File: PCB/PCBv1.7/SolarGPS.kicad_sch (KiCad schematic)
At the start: 38 parts, among them J1 Conn_01x10_Female, J2 GND, J3 GND, J4 Solar1+, J5 Solar2+, J6 Conn_02x03_Odd_Even, J7 Screw_Terminal_01x01, J8 Conn_01x04_Male, SW1 SW_Push, U1 TPS63802, U2 SAM-M10Q, U3 STM32L071KBTx, U4 MAX40200AUK, Y1 32.768

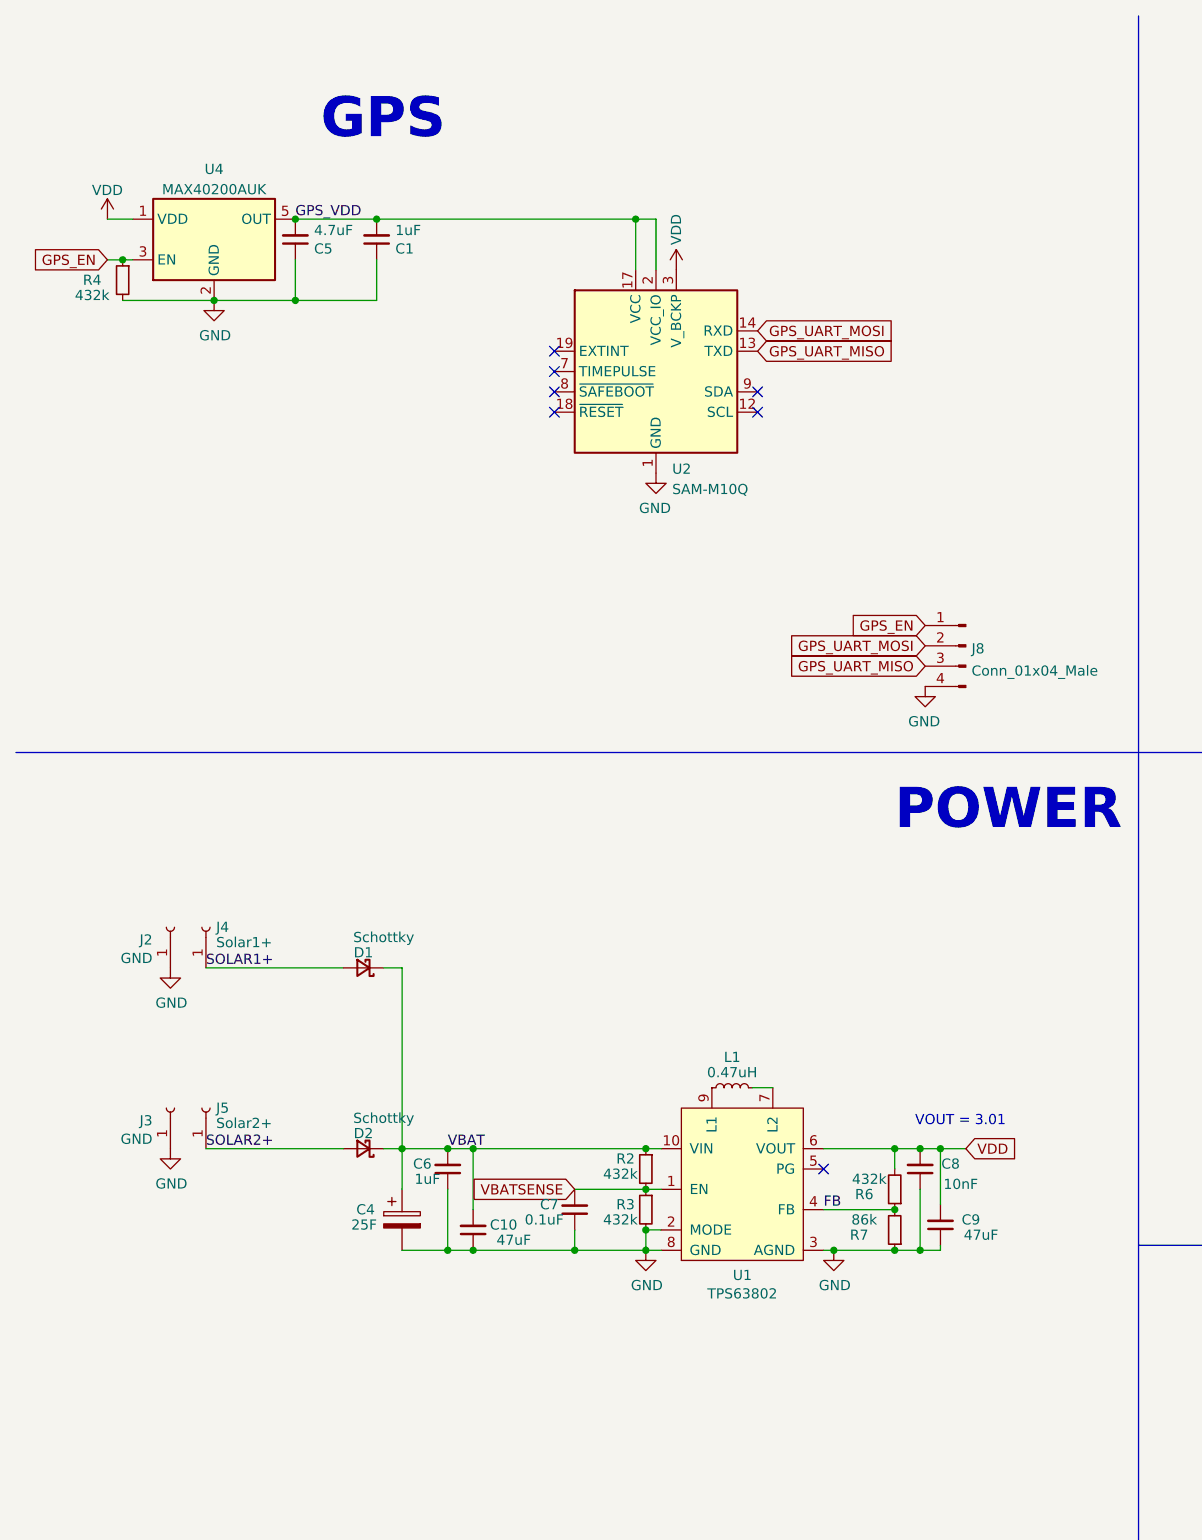
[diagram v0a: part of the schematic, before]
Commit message: Submit board 1.7
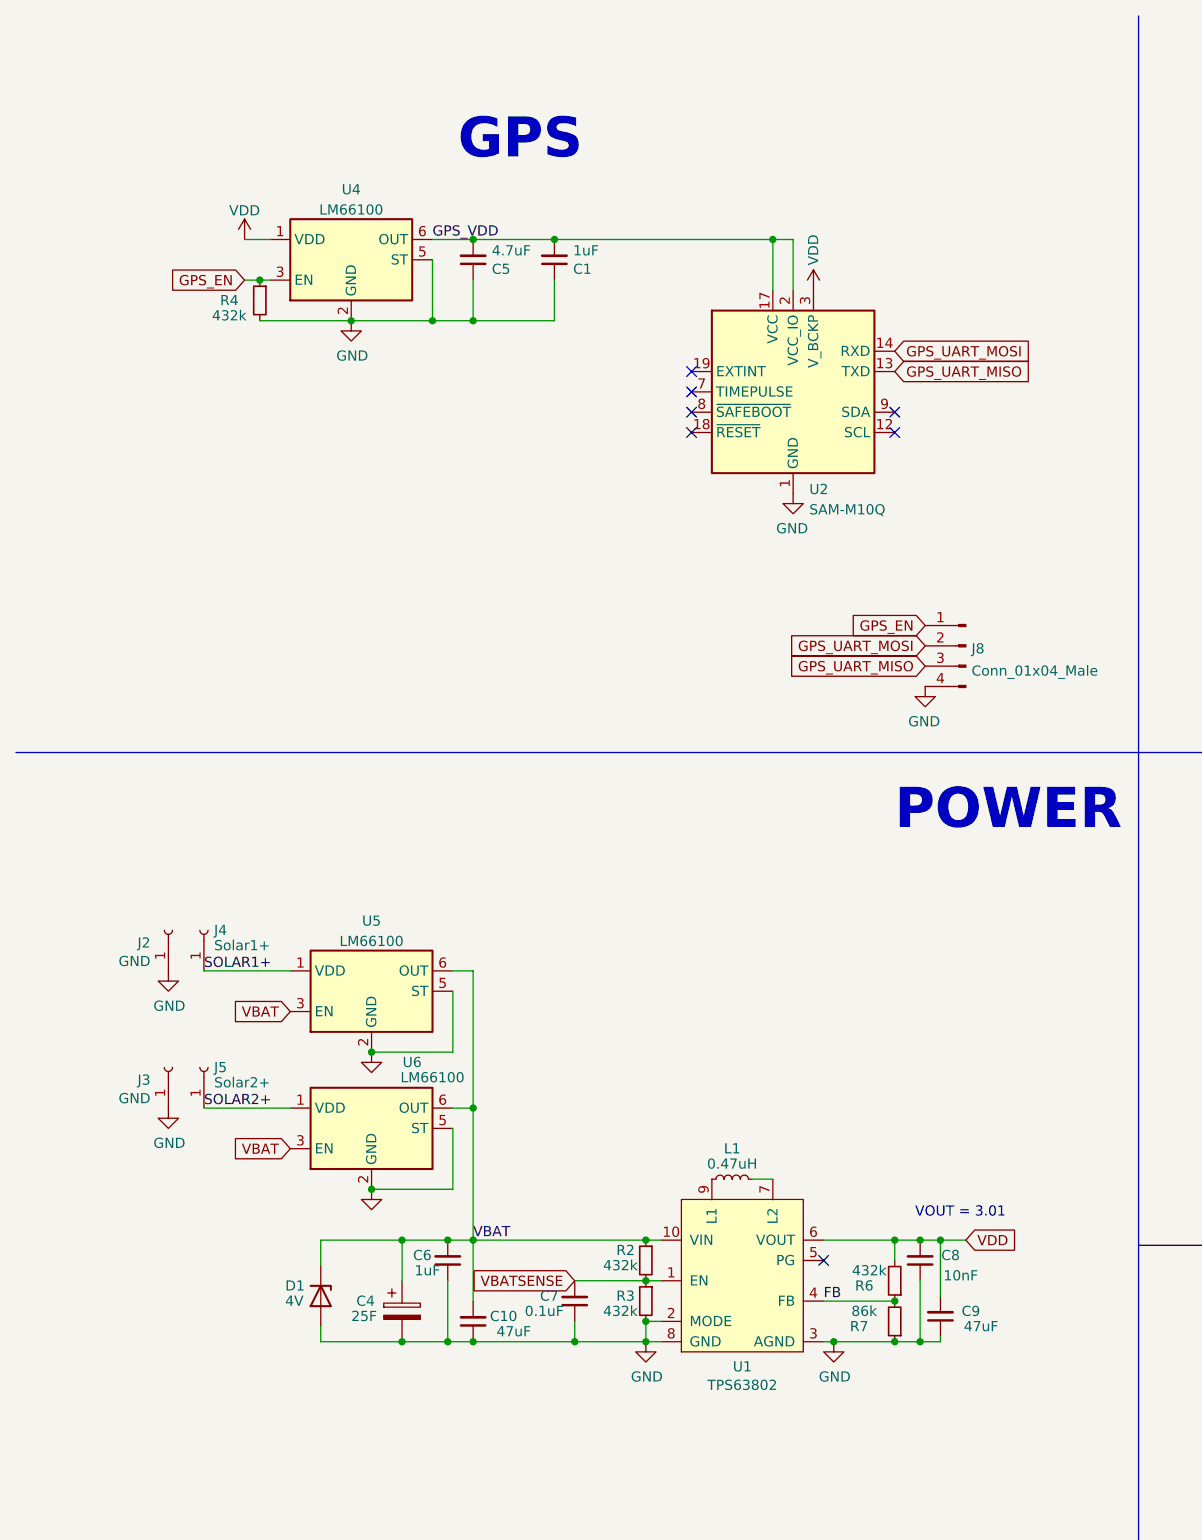
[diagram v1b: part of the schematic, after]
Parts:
- removed D1, D2: Schottky, Diode_SMD:D_SOD-323_HandSoldering, symbol Device:D_Schottky_Small
- removed U4: MAX40200AUK, Package_TO_SOT_SMD:SOT-23-5, symbol Analog_Switch:MAX40200AUK
- added D1: 4V, Diode_SMD:D_SMB_Handsoldering, symbol Device:D_Zener
- added U4, U5, U6: LM66100, Package_TO_SOT_SMD:SOT-363_SC-70-6, symbol Heliograph:LM66100
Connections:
- net GND: now also D1.2 (A), U4.2 (GND), U4.5 (ST), U5.2 (GND), U5.5 (ST), U6.2 (GND), U6.5 (ST)
- net GPS_EN: now also U4.3 (EN)
- net GPS_VDD: now also U4.6 (OUT)
- net SOLAR1+: now also U5.1 (VDD)
- net SOLAR2+: now also U6.1 (VDD)
- net VBAT: now also D1.1 (K), U5.3 (EN), U5.6 (OUT), U6.3 (EN), U6.6 (OUT)
- net VDD: now also U4.1 (VDD)
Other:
- moved on the sheet: C1, C10, C4, C5, C6, C7, C8, C9, J3, J5, L1, R2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
